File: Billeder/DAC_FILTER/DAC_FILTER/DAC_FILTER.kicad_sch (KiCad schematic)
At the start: 66 parts, among them U1 LTC1668, U2 OPA4830, U3 OPA4830

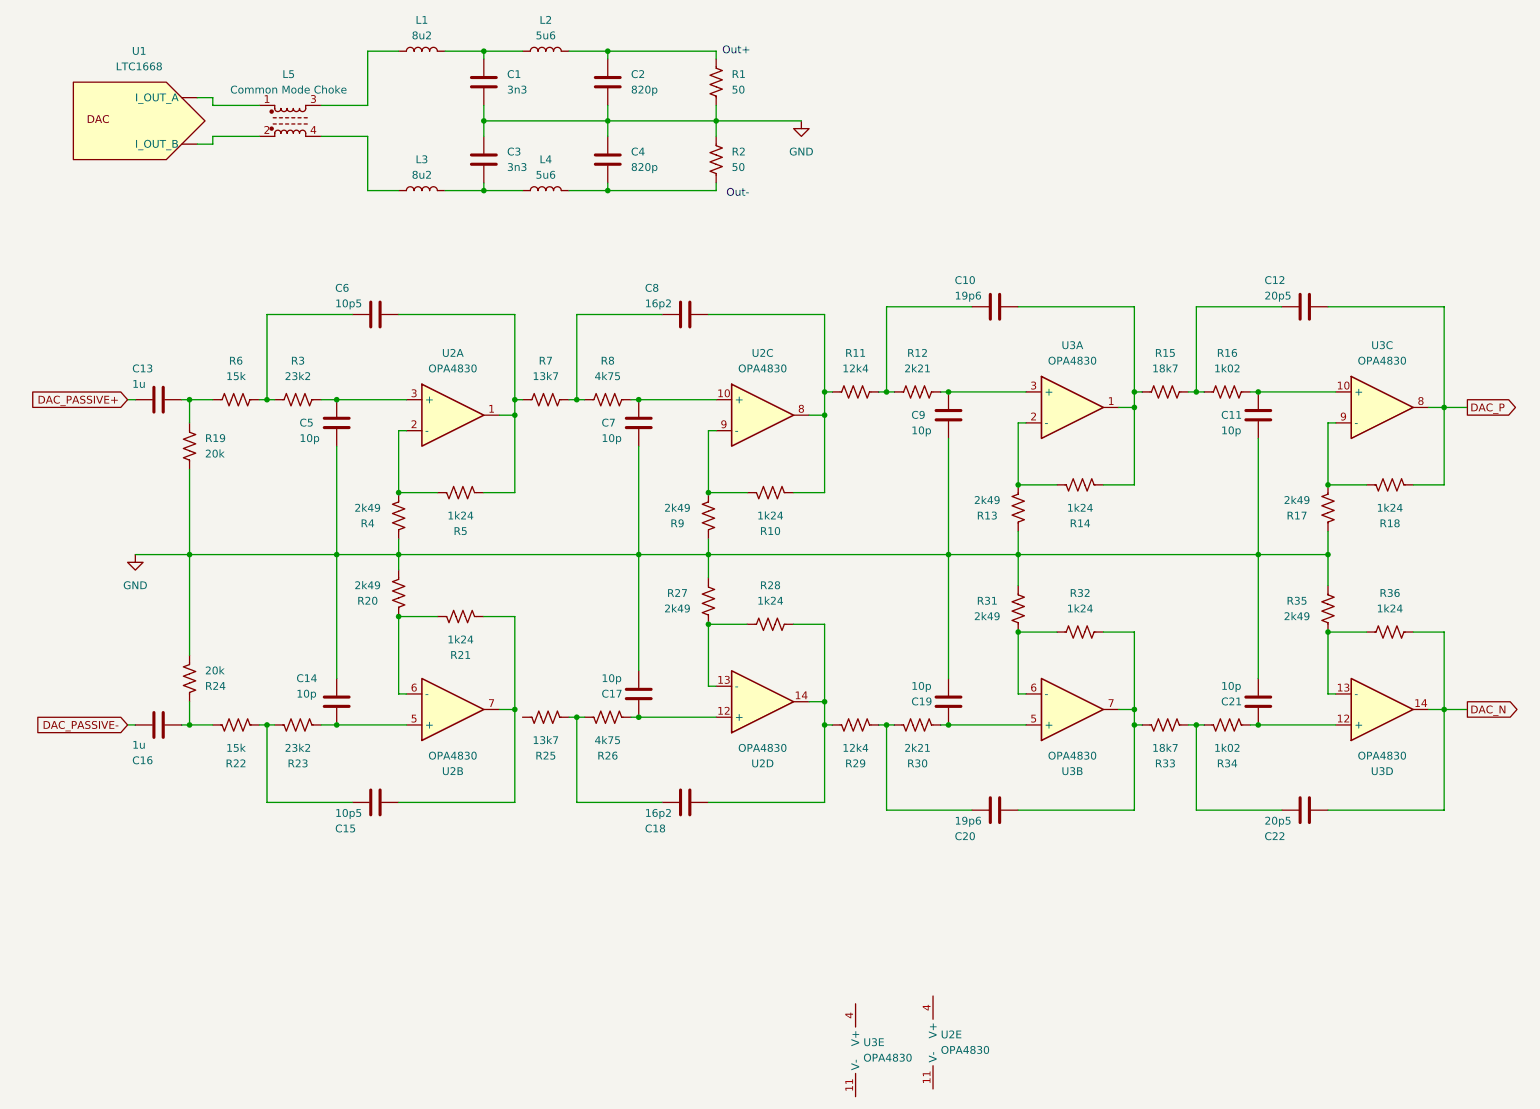
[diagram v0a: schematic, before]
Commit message: DC power amp calculations
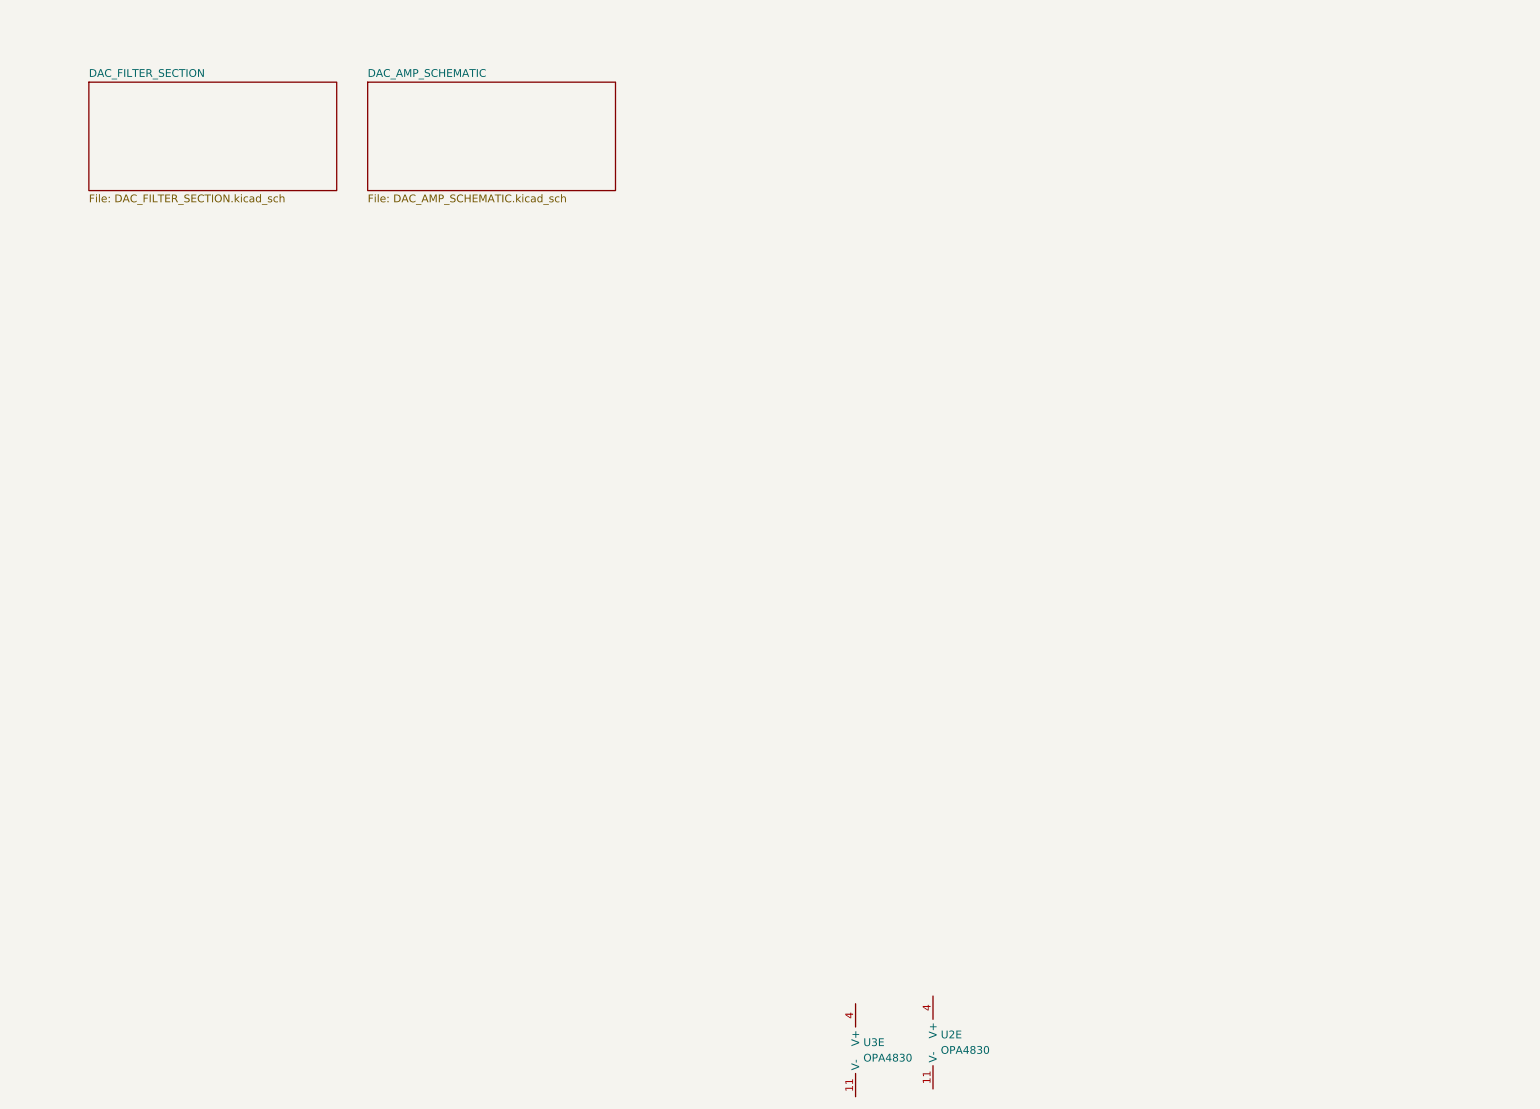
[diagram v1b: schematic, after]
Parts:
- removed C1, C3: 3n3, symbol Device:C
- removed C10, C20: 19p6, symbol Device:C
- removed C11, C14, C17, C19, C21, C5, C7, C9: 10p, symbol Device:C
- removed C12, C22: 20p5, symbol Device:C
- removed C13, C16: 1u, symbol Device:C
- removed C15, C6: 10p5, symbol Device:C
- removed C18, C8: 16p2, symbol Device:C
- removed C2, C4: 820p, symbol Device:C
- removed L1, L3: 8u2, symbol Device:L
- removed L2, L4: 5u6, symbol Device:L
- removed L5: Common Mode Choke, symbol Device:L_Ferrite_Coupled_1324
- removed R1, R2: 50, symbol Device:R_US
- removed R10, R14, R18, R21, R28, R32, R36, R5: 1k24, symbol Device:R_US
- removed R11, R29: 12k4, symbol Device:R_US
- removed R12, R30: 2k21, symbol Device:R_US
- removed R13, R17, R20, R27, R31, R35, R4, R9: 2k49, symbol Device:R_US
- removed R15, R33: 18k7, symbol Device:R_US
- removed R16, R34: 1k02, symbol Device:R_US
- removed R19, R24: 20k, symbol Device:R_US
- removed R22, R6: 15k, symbol Device:R_US
- removed R23, R3: 23k2, symbol Device:R_US
- removed R25, R7: 13k7, symbol Device:R_US
- removed R26, R8: 4k75, symbol Device:R_US
- removed U1: LTC1668, symbol JFT_DAC:LTC1668
- removed unit 4 of U2
- removed unit 1 of U2
- removed unit 2 of U2
- removed unit 3 of U2
- removed unit 2 of U3
- removed unit 1 of U3
- removed unit 3 of U3
- removed unit 4 of U3
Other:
- added sheet DAC_AMP_SCHEMATIC (DAC_AMP_SCHEMATIC.kicad_sch)
- added sheet DAC_FILTER_SECTION (DAC_FILTER_SECTION.kicad_sch)
- note removed: "Out+"
- note removed: "Out-"
